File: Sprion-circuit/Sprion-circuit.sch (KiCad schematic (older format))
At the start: 0 parts

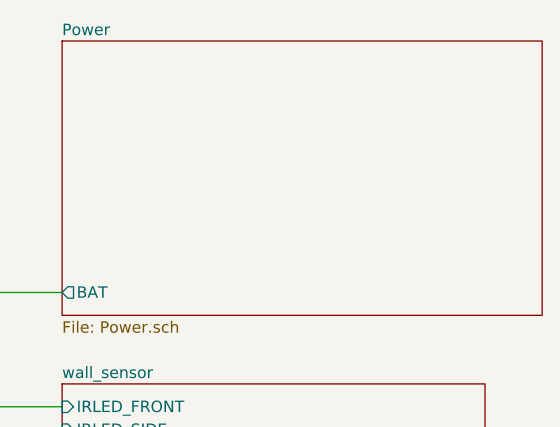
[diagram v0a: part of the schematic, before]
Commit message: add,feat,fix:すまんコミットわすれててぐちゃぐちゃや
配置始めた。
フットプリント割り当てた
回路図pdfで吐いた
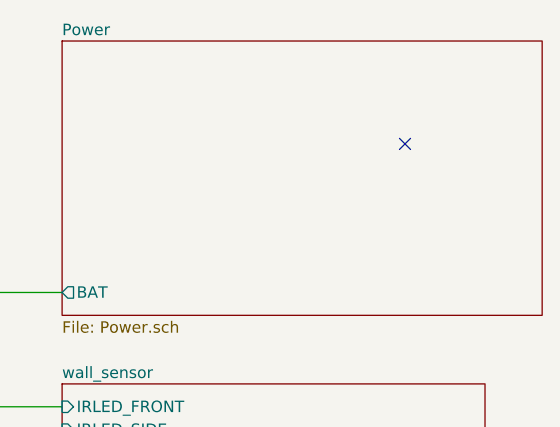
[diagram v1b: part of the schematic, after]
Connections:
- no-connect marks 0 -> 1
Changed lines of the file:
@@
 Wire Wire Line
 	5200 3400 4400 3400
+NoConn ~ 10000 2050
 $EndSCHEMATC

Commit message: add fix feat: でけたー（コミットしてなくてごめん）
ベタ塗、配線、再配置等
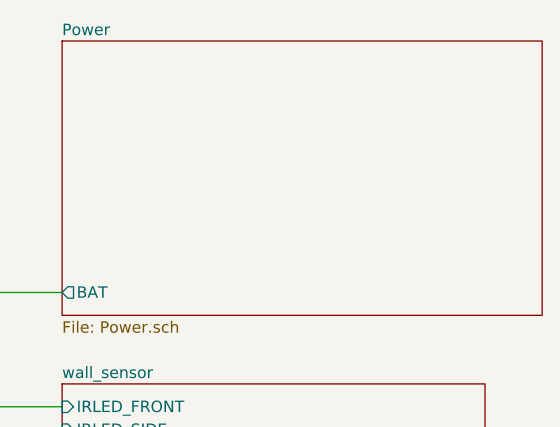
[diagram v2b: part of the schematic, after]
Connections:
- no-connect marks 1 -> 0
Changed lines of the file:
@@
 $EndDescr
-$Sheet
-S 8500 1600 2100 1200
-U 60F3852A
-F0 "Power" 50
-F1 "Power.sch" 50
-F2 "BAT" O L 8500 2700 50
-$EndSheet
 $Sheet
 S 8500 3100 1850 900
@@
 Wire Wire Line
 	5200 3400 4400 3400
-NoConn ~ 10000 2050
+$Sheet
+S 8500 1600 2100 1200
+U 60F3852A
+F0 "Power" 50
+F1 "Power.sch" 50
+F2 "BAT" O L 8500 2700 50
+$EndSheet
 $EndSCHEMATC
